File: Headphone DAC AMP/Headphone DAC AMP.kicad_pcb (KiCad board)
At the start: 4 copper layers, 35 x 71 mm, 96 parts, among them J1 2137160001, J2 M50-3551042, J4 PINHD_1x2_Male, U1 NCV8187AMTW090TAG, U11 ADP5071AREZ-R7, U2 XU316-1024-QF60B-C24, U6 MCP1727-1802xSN, U7 MCP1727-3302xSN, U8 W25Q16JVSNIQ, Y1 Crystal_GND24, Y2 LMK6CE049152CDLFR, Y3 ASDLJ-E-45.1584MHz

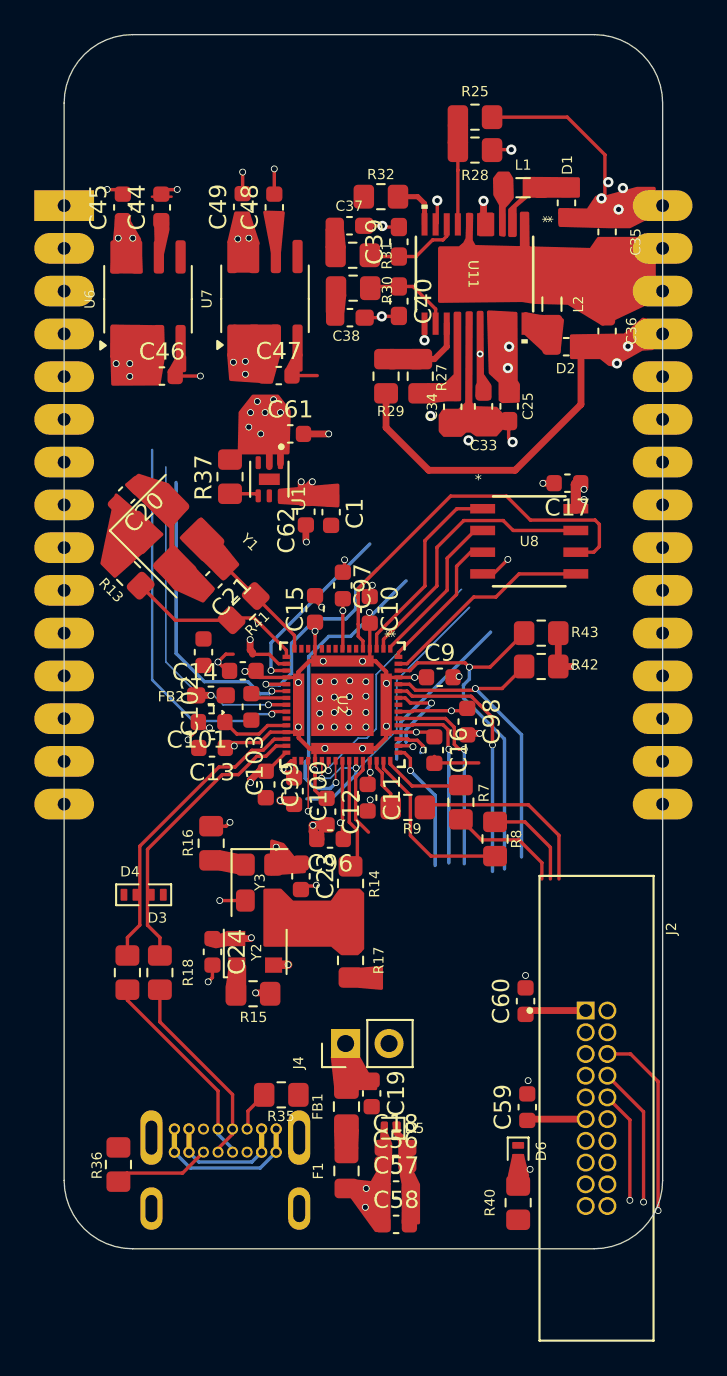
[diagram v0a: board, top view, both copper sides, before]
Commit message: messed with the layouts a bit
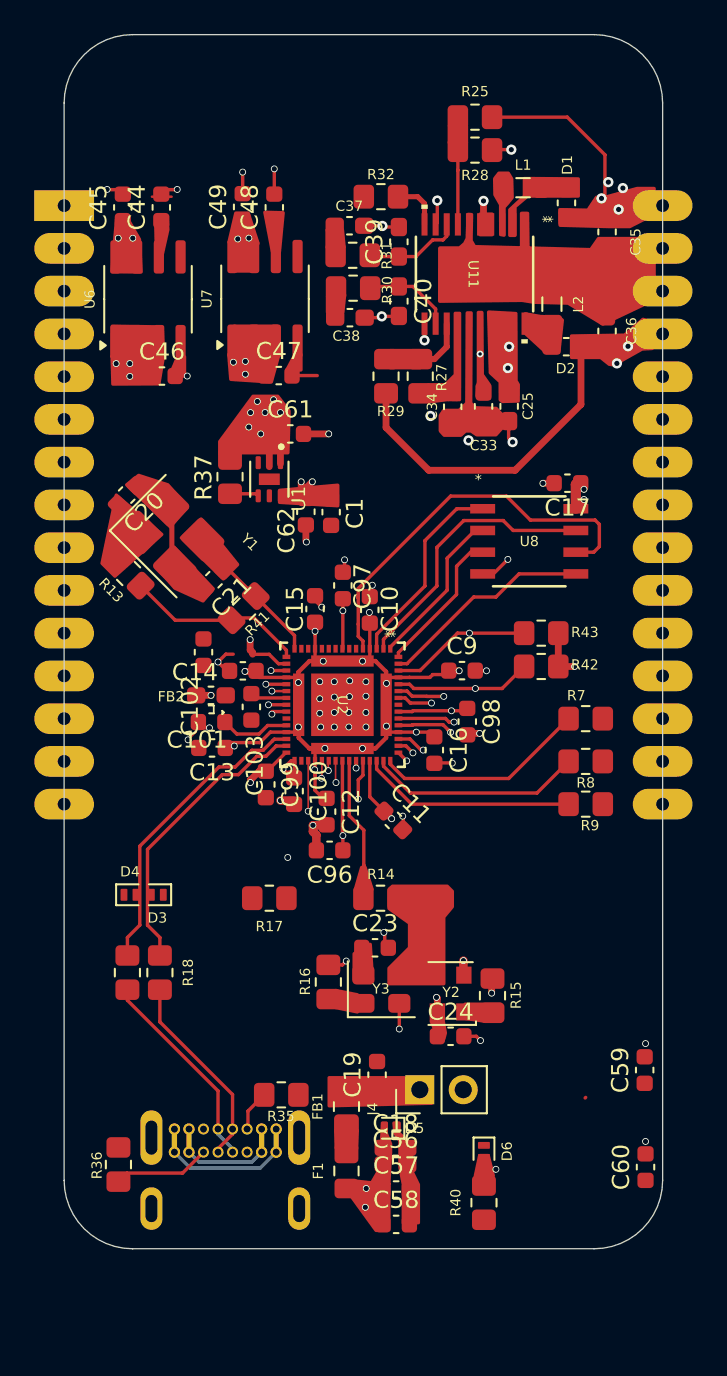
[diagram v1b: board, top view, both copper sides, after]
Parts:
- removed J2: M50-3551042, M50_3551042:HARWIN_M50-3551042
- moved C24 14.8 mm to (103.4, 137.5), turned to 0 degrees
- moved R15 14.0 mm to (105.9, 135.1), turned to -90 degrees
- moved C60 12.0 mm to (114.8, 145.1)
- moved Y2 11.7 mm to (103.4, 135.0), turned to 180 degrees
- moved R16 10.6 mm to (96.3, 134.3)
- moved R9 10.4 mm to (111.3, 123.9)
- moved Y3 9.47 mm to (99.4, 134.7), turned to 0 degrees
- moved R7 8.79 mm to (111.3, 118.9), turned to 0 degrees
- moved C59 7.20 mm to (114.8, 139.4)
- moved R8 6.98 mm to (111.3, 121.4), turned to 0 degrees
- moved C23 6.02 mm to (99.0, 132.3), turned to 0 degrees
- moved R17 5.98 mm to (92.8, 129.4), turned to 180 degrees
- moved J4 5.11 mm to (101.6, 140.6)
- moved C11 2.01 mm to (100.1, 124.9), turned to -45 degrees
- moved D6 2.00 mm to (105.4, 144.2)
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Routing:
- net /Debug/XMOS_NRST: track 24.3 -> 1.11 mm, vias 3 -> 2
- net /Debug/TDO: track 23.4 -> 1.20 mm, vias 2 -> 1
- net /Debug/TCK: track 22.5 -> 0.85 mm
- net /Debug/TMS: track 19.3 -> 0.85 mm
- net /Debug/TDI: track 18.9 -> 0.85 mm, vias 2 -> 1
- net /Debug/4D3: track 18.3 -> 1.29 mm
- net /Debug/4D1: track 15.4 -> 0.85 mm
- net /Debug/4D2: track 14.7 -> 0.59 mm
- net /USB Audio Input/SDA: track 21.4 -> 8.26 mm
- net /USB Audio Input/DAC_GP6: track 15.1 -> 2.62 mm
- net /USB Audio Input/SCL: track 19.0 -> 7.99 mm
- net unconnected-(R9-Pad2): track 10.9 -> 0.00 mm
- net /Debug/4D0: track 12.7 -> 2.95 mm
- net /USB Audio Input/BCLK: track 3.74 -> 12.6 mm
- net /USB Audio Input/DAC_GP5: track 11.9 -> 3.24 mm
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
